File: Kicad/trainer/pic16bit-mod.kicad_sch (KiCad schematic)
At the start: 23 parts, among them K301 I2C/GPIO, K303 SPI/GPIO, K304 EUSART/TTL

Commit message: Up
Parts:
- K301, K304: symbol tronixio:SAMTEC-SSW-106-02-T-S-RA -> tronixio:SAMTEC-254-F-1X06-RIGHT-ANGLE; Mouser 200-SSW10602TSRA -> 200-SSW10603TSRA
- K303: symbol tronixio:SAMTEC-SSW-106-02-T-D-RA -> tronixio:SAMTEC-254-F-2X06-RIGHT-ANGLE
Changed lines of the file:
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@@
 	)
 	(symbol
-		(lib_id "tronixio:SAMTEC-SSW-106-02-T-S-RA")
+		(lib_id "tronixio:SAMTEC-254-F-1X06-RIGHT-ANGLE")
 		(at 241.3 43.18 0)
 		(unit 1)
@@
 			)
 		)
-		(property "Mouser" "200-SSW10602TSRA"
+		(property "Mouser" "200-SSW10603TSRA"
 			(at 241.3 66.04 0)
 			(effects
@@
 	)
 	(symbol
-		(lib_id "tronixio:SAMTEC-SSW-106-02-T-S-RA")
+		(lib_id "tronixio:SAMTEC-254-F-1X06-RIGHT-ANGLE")
 		(at 104.14 43.18 0)
 		(unit 1)
@@
 			)
 		)
-		(property "Mouser" "200-SSW10602TSRA"
+		(property "Mouser" "200-SSW10603TSRA"
 			(at 104.14 66.04 0)
 			(effects
@@
 	)
 	(symbol
-		(lib_id "tronixio:SAMTEC-SSW-106-02-T-D-RA")
+		(lib_id "tronixio:SAMTEC-254-F-2X06-RIGHT-ANGLE")
 		(at 139.7 124.46 0)
 		(unit 1)

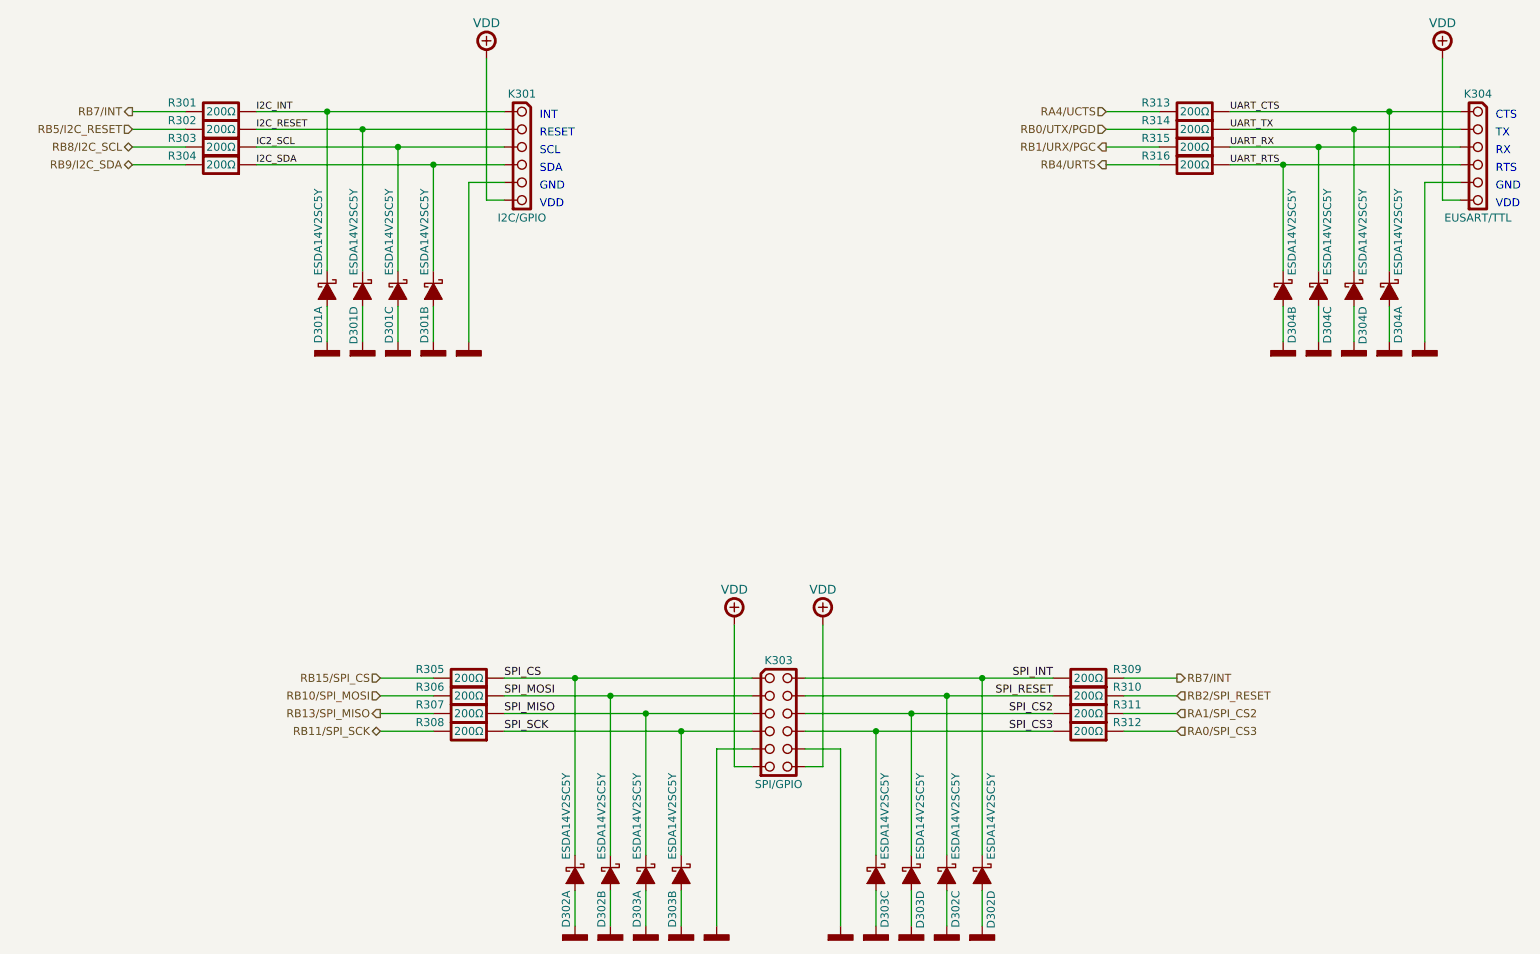
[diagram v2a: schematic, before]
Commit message: Up
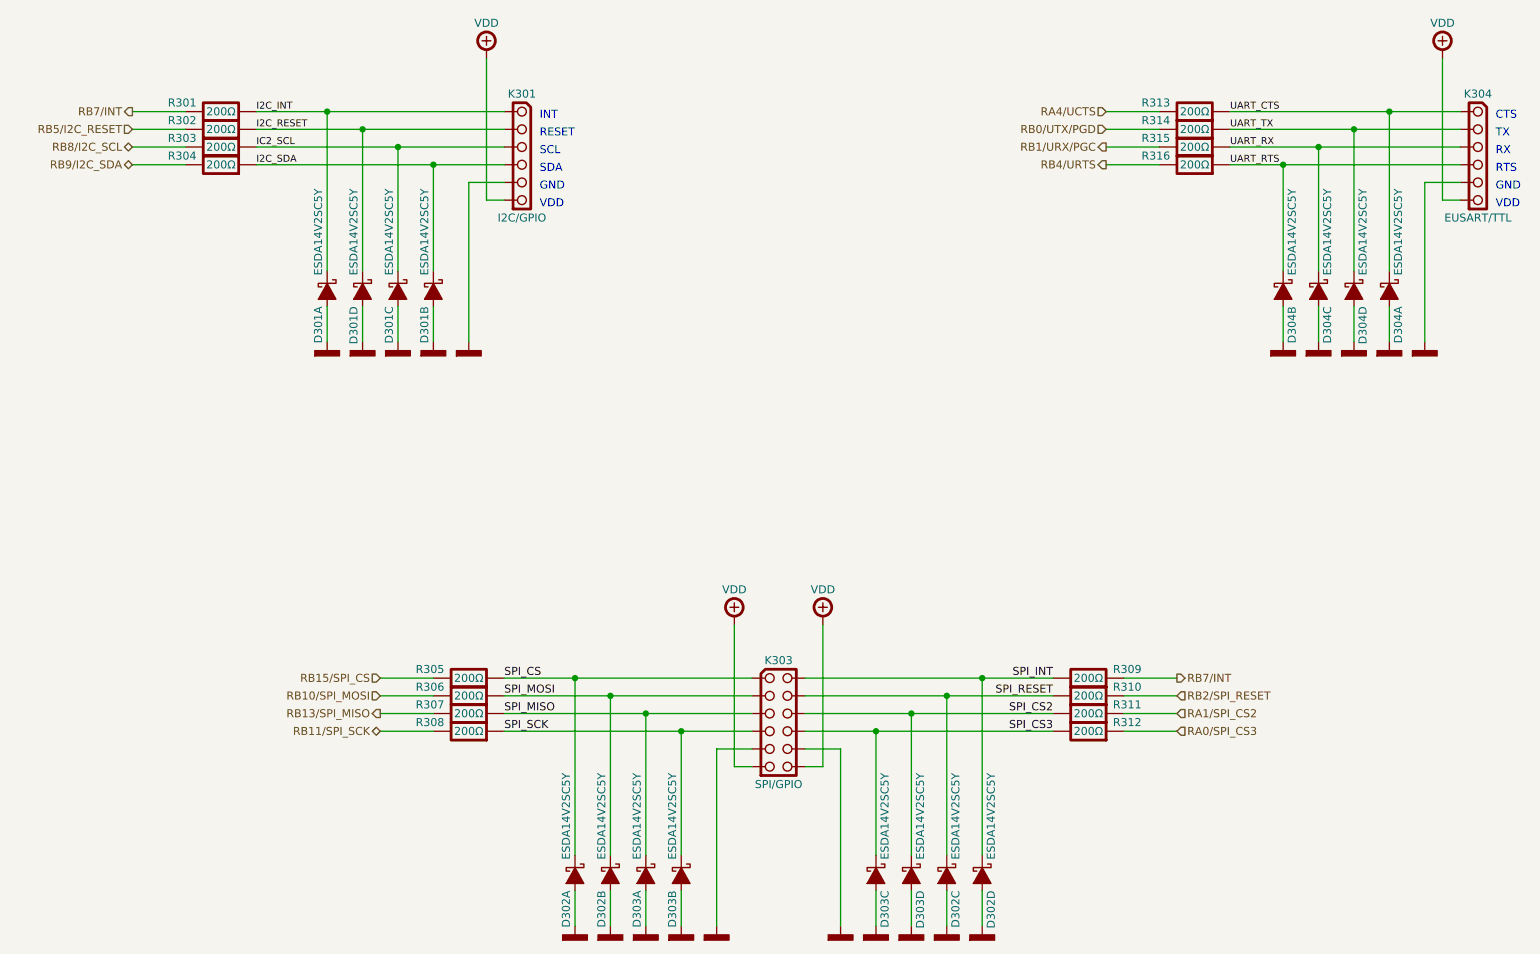
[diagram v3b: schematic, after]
